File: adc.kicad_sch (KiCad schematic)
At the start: 24 parts, among them U70 AD7177-2BRUZ, U75 OPA2189D

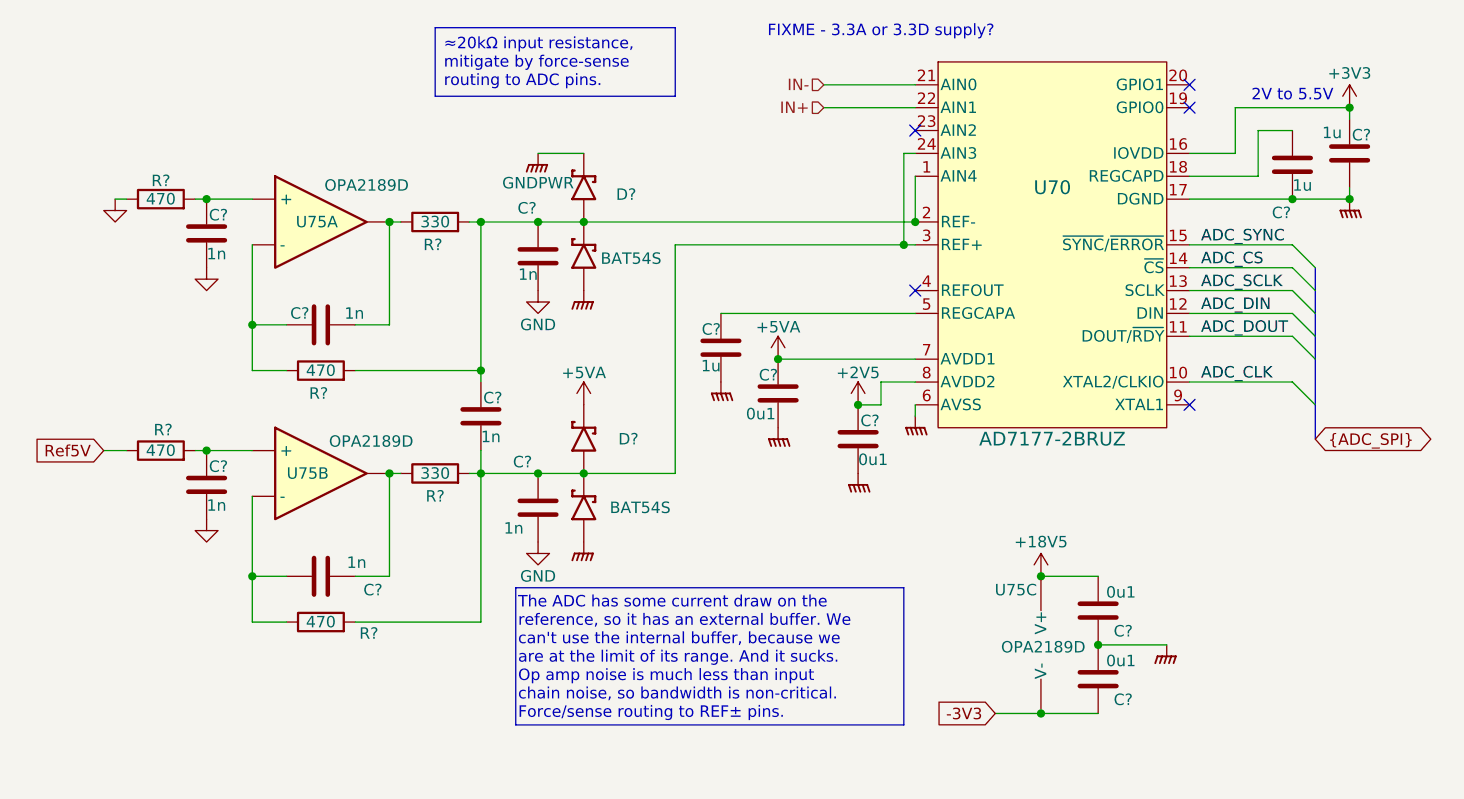
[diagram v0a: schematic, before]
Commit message: Schematic complete, maybe
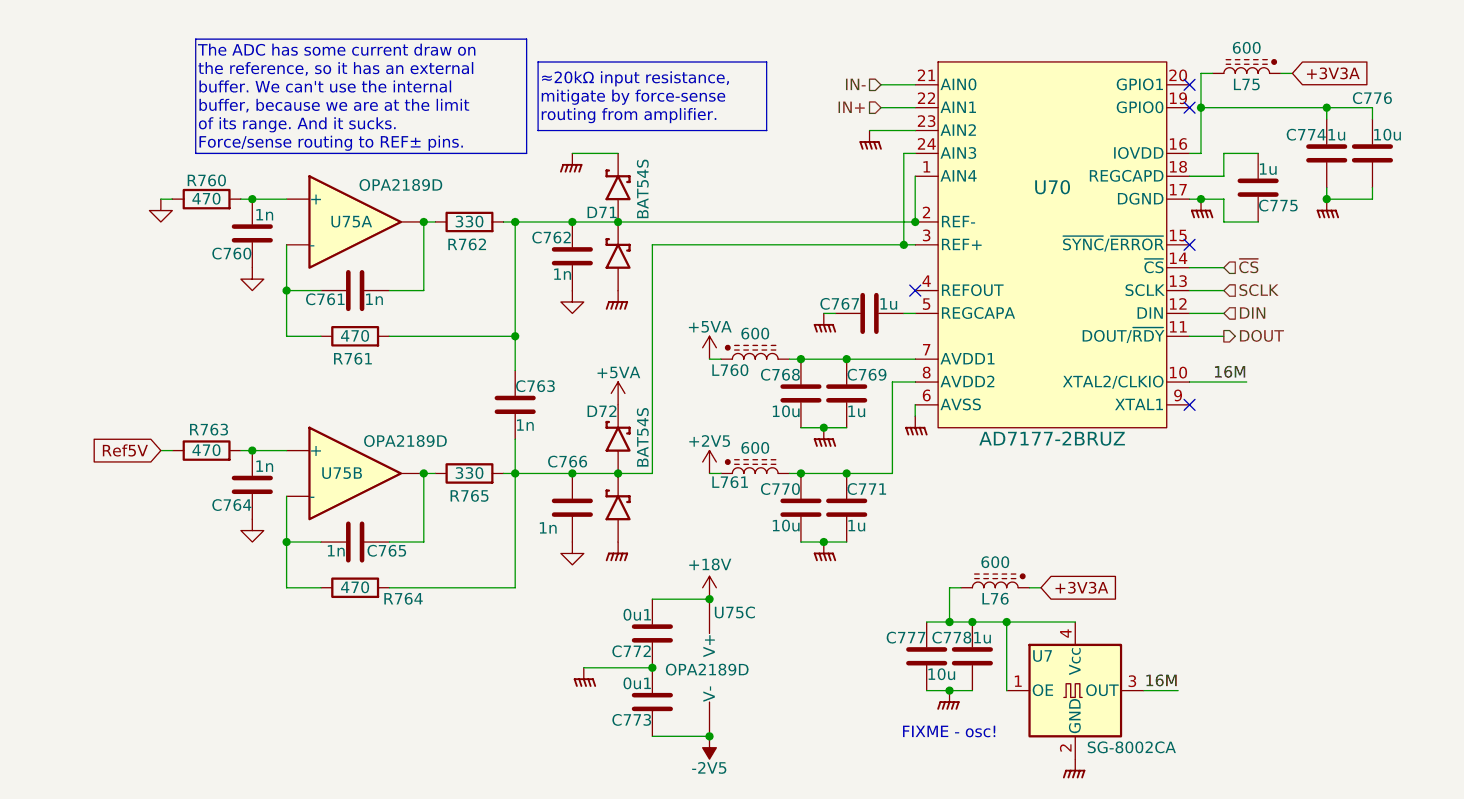
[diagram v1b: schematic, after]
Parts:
- added C768, C770, C776, C777: 10u, Capacitor_SMD:C_0603_1608Metric, symbol Device:C
- added C778: 1u, Capacitor_SMD:C_0402_1005Metric, symbol Device:C
- added L75, L76, L760, L761: 600, Inductor_SMD:L_0603_1608Metric, symbol Parts:L_Ferrite_Power
- added U7: SG-8002CA, Oscillator:Oscillator_SMD_SeikoEpson_SG8002CA-4Pin_7.0x5.0mm, symbol Oscillator:SG-8002CA
- C767, C774, C775: renamed from C?; LCSC (none) -> C52923
- C769, C771: renamed from C?; value 0u1 -> 1u; LCSC (none) -> C52923
- C772, C773: renamed from C?; LCSC (none) -> C307331
- U70: now left out of the parts list
- U75: LCSC (none) -> C881489; now left out of the parts list
- gave numbers to parts that had none: 15
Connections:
- net +2V5: now also L761.1; no longer C771.1, U70.8 (AVDD2)
- net +5VA: now also L760.1; no longer C769.1, U70.7 (AVDD1)
- net GNDPWR: now also U70.23 (AIN2), C768.2, C770.2, C776.2, C777.2, C778.2, U7.2 (GND)
- net +18V5 renamed +18V
- net +3V3: no longer names the net of C774.1, U70.16 (IOVDD)
- net +3V3: now also C776.1, L75.2
- net -3V3 renamed -2V5
- net ADC_CLK renamed 16M
- net 16M: now also U7.3 (OUT)
- net ADC_CS renamed ~{CS}
- net ADC_DIN renamed DIN
- net ADC_DOUT renamed DOUT
- net ADC_SCLK renamed SCLK
- net ADC_SYNC: no longer names the net of U70.15 (~{SYNC}/~{ERROR})
- new net: C768.1, C769.1, L760.2, U70.7 (AVDD1)
- new net: C777.1, C778.1, L76.2, U7.1 (OE), U7.4 (Vcc)
- new net: C770.1, C771.1, L761.2, U70.8 (AVDD2)
- new net +3V3A: L75.1, L76.1
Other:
- note added: "FIXME - osc!"
- note removed: "2V to 5.5V"
- note removed: "FIXME - 3.3A or 3.3D supply?"
- moved on the sheet: C760, C761, C762, C763, C764, C765, C766, C767, C769, C771, C772, C773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
